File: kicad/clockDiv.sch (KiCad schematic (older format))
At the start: 2 parts

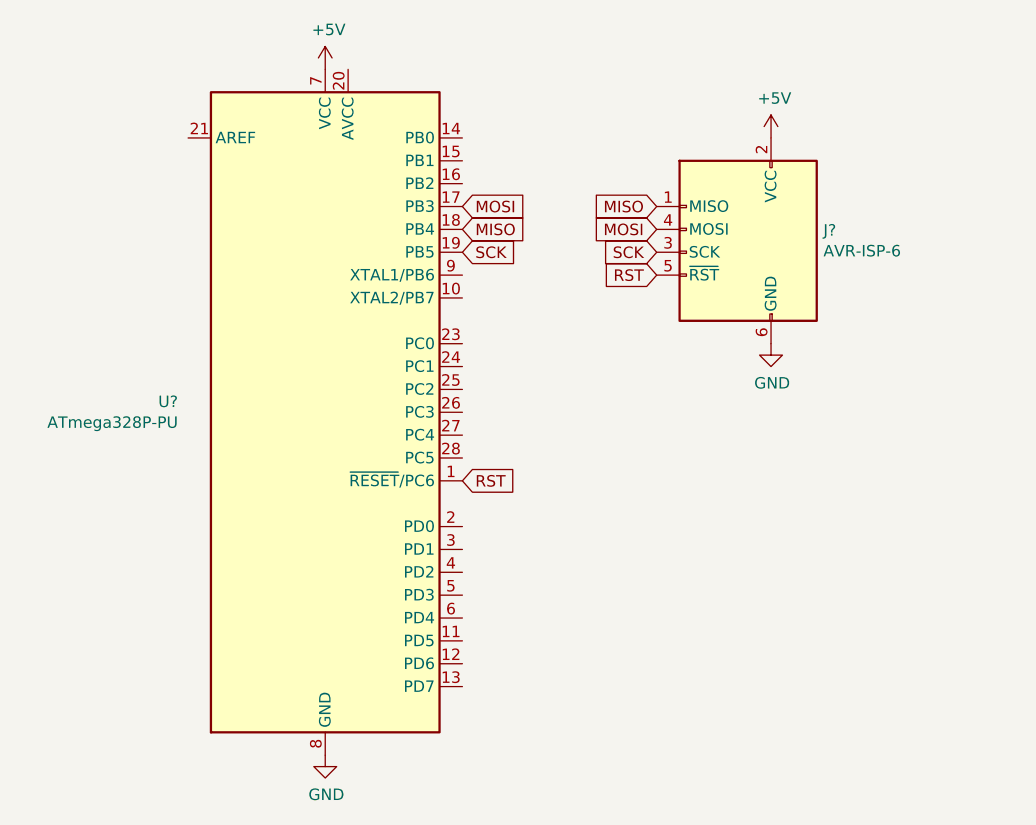
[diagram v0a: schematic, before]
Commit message: add crystal
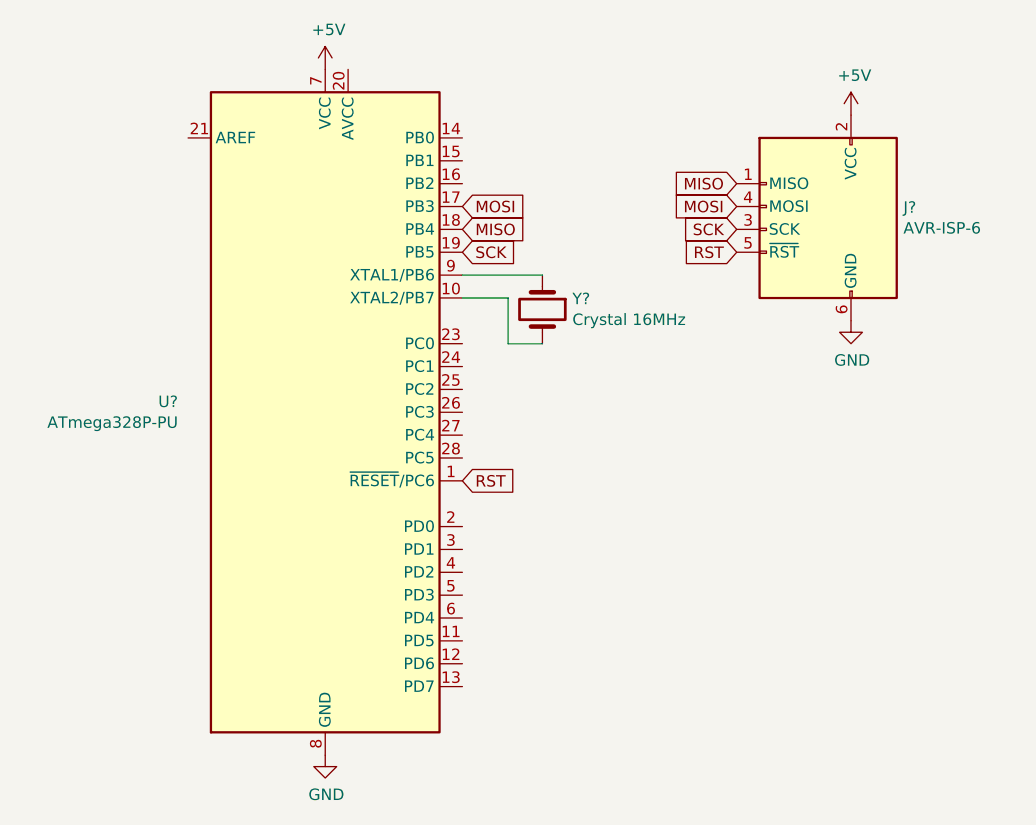
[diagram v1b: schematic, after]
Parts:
- added Y?: Crystal 16MHz, symbol Device:Crystal
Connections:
- net at U?.10 (XTAL2/PB7): now also Y?.2
- net at U?.9 (XTAL1/PB6): now also Y?.1
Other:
- moved on the sheet: J?
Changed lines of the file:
@@
 L Connector:AVR-ISP-6 J?
 U 1 1 5EFE5F5A
-P 7000 3100
-F 0 "J?" H 6671 3196 50  0000 R CNN
-F 1 "AVR-ISP-6" H 6671 3105 50  0000 R CNN
-F 2 "" V 6750 3150 50  0001 C CNN
-F 3 " ~" H 5725 2550 50  0001 C CNN
-	1    7000 3100
+P 7350 3000
+F 0 "J?" H 7021 3096 50  0000 R CNN
+F 1 "AVR-ISP-6" H 7021 3005 50  0000 R CNN
+F 2 "" V 7100 3050 50  0001 C CNN
+F 3 " ~" H 6075 2450 50  0001 C CNN
+	1    7350 3000
 	-1   0    0    -1
 $EndComp
@@
 L power:GND #PWR?
 U 1 1 5EFF1BEB
-P 7100 3500
-F 0 "#PWR?" H 7100 3250 50  0001 C CNN
-F 1 "GND" H 7105 3327 50  0000 C CNN
-F 2 "" H 7100 3500 50  0001 C CNN
-F 3 "" H 7100 3500 50  0001 C CNN
-	1    7100 3500
+P 7450 3400
+F 0 "#PWR?" H 7450 3150 50  0001 C CNN
+F 1 "GND" H 7455 3227 50  0000 C CNN
+F 2 "" H 7450 3400 50  0001 C CNN
+F 3 "" H 7450 3400 50  0001 C CNN
+	1    7450 3400
 	1    0    0    -1
 $EndComp
@@
 L power:+5V #PWR?
 U 1 1 5EFF32A5
-P 7100 2600
-F 0 "#PWR?" H 7100 2450 50  0001 C CNN
-F 1 "+5V" H 7115 2773 50  0000 C CNN
-F 2 "" H 7100 2600 50  0001 C CNN
-F 3 "" H 7100 2600 50  0001 C CNN
-	1    7100 2600
+P 7450 2500
+F 0 "#PWR?" H 7450 2350 50  0001 C CNN
+F 1 "+5V" H 7465 2673 50  0000 C CNN
+F 2 "" H 7450 2500 50  0001 C CNN
+F 3 "" H 7450 2500 50  0001 C CNN
+	1    7450 2500
 	1    0    0    -1
 $EndComp
 Text GLabel 5750 3100 2    50   Input ~ 0
 SCK
-Text GLabel 6600 3100 0    50   Input ~ 0
+Text GLabel 6950 3000 0    50   Input ~ 0
 SCK
 Text GLabel 5750 3000 2    50   Input ~ 0
 MISO
-Text GLabel 6600 2900 0    50   Input ~ 0
+Text GLabel 6950 2800 0    50   Input ~ 0
 MISO
 Text GLabel 5750 2900 2    50   Input ~ 0
 MOSI
-Text GLabel 6600 3000 0    50   Input ~ 0
+Text GLabel 6950 2900 0    50   Input ~ 0
 MOSI
 Text GLabel 5750 4100 2    50   Input ~ 0
 RST
-Text GLabel 6600 3200 0    50   Input ~ 0
+Text GLabel 6950 3100 0    50   Input ~ 0
 RST
+$Comp
+L Device:Crystal Y?
+U 1 1 5EFE63D4
+P 6100 3350
+F 0 "Y?" V 6054 3481 50  0000 L CNN
+F 1 "Crystal 16MHz" V 6145 3481 50  0000 L CNN
+F 2 "" H 6100 3350 50  0001 C CNN
+F 3 "~" H 6100 3350 50  0001 C CNN
+	1    6100 3350
+	0    1    1    0
+$EndComp
+Wire Wire Line
+	6100 3200 5750 3200
+Wire Wire Line
+	6100 3500 5950 3500
+Wire Wire Line
+	5950 3500 5950 3300
+Wire Wire Line
+	5950 3300 5750 3300
 $EndSCHEMATC
